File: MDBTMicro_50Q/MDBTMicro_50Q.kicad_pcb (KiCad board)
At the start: 2 copper layers, 33 x 18 mm, 24 parts, among them J1 USB_C_Receptacle_USB2.0, J2 SWD, U1 XC6220B331MR-G, U2 TP4057, U3 MDBT50Q-x1MV2, U4 ProMicro, X1 32.768kHz

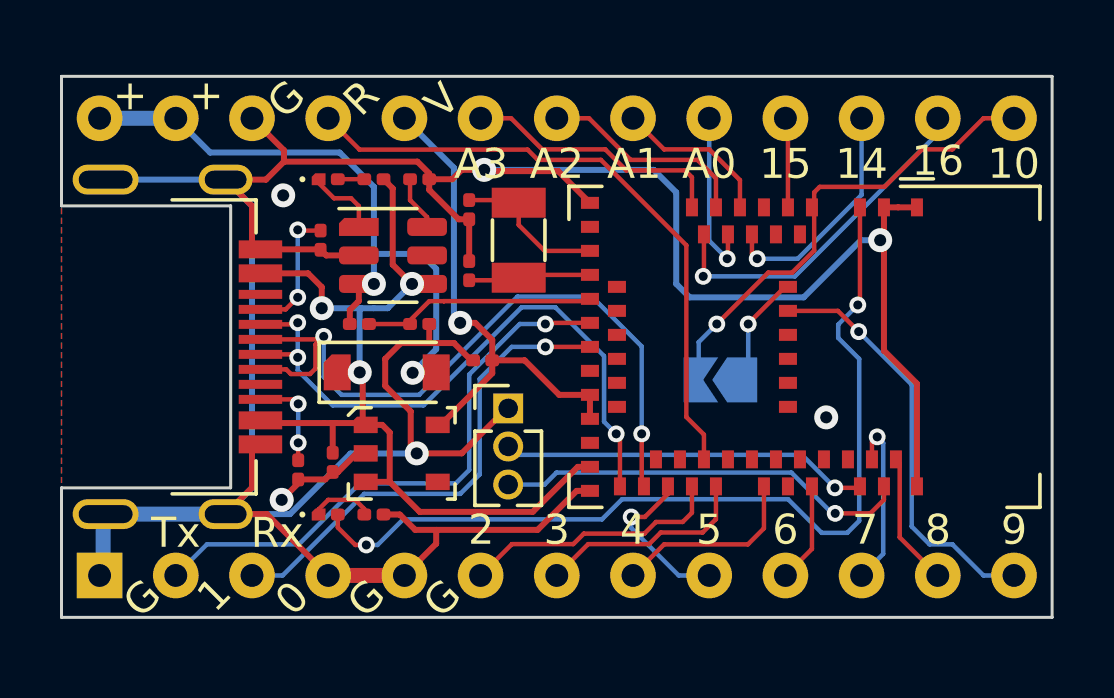
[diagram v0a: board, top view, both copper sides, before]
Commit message: Update footprint
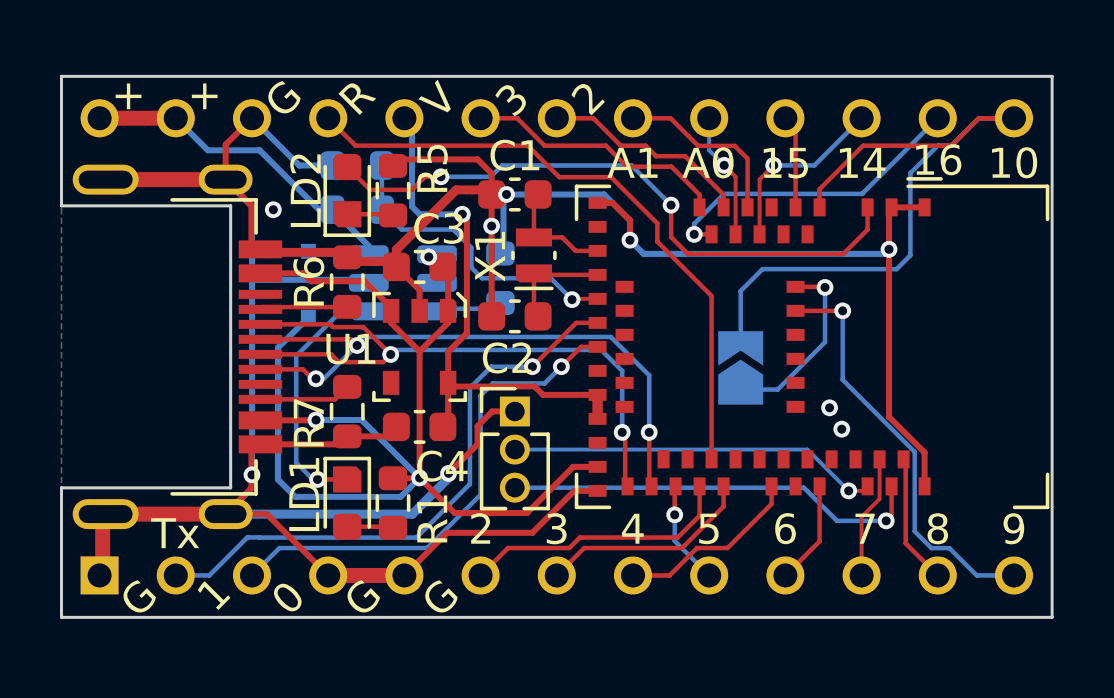
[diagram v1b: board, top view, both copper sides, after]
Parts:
- C1, C2, C3, C4: footprint Capacitor_SMD:C_0201_0603Metric -> Capacitor_SMD:C_0603_1608Metric
- D1: footprint Diode_SMD:D_SOD-123 -> Diode_SMD:D_SOD-323F; moved to B.Cu
- LD1: value RED -> Charging; footprint LED_SMD:LED_0201_0603Metric -> LED_SMD:LED_0603_1608Metric
- LD2: value BLUE -> User; footprint LED_SMD:LED_0201_0603Metric -> LED_SMD:LED_0603_1608Metric
- R1, R5, R6, R7: footprint Resistor_SMD:R_0201_0603Metric -> Resistor_SMD:R_0603_1608Metric
- R2, R3, R4: footprint Resistor_SMD:R_0201_0603Metric -> Resistor_SMD:R_0603_1608Metric; moved to B.Cu
- U2: moved to B.Cu
- X1: footprint Crystal:Crystal_SMD_3215-2Pin_3.2x1.5mm -> Crystal:Crystal_SMD_MicroCrystal_CM9V-T1A-2Pin_1.6x1.0mm
- moved LD1 10.8 mm to (140.3, 106.8), turned to -90 degrees
- moved LD2 10.8 mm to (140.3, 96.4), turned to 90 degrees
- moved R1 10.8 mm to (141.9, 106.8), turned to 90 degrees
- moved R5 10.8 mm to (141.9, 96.4), turned to -90 degrees
- moved C3 7.13 mm to (142.7, 98.9), turned to 0 degrees
- moved R4 5.68 mm to (140.7, 95.6), turned to 0 degrees
- moved R2 4.26 mm to (145.4, 99.3), turned to -90 degrees
- moved D1 3.93 mm to (139.0, 99.5), turned to 90 degrees
- moved R3 3.81 mm to (140.7, 97.0)
- moved U1 3.60 mm to (142.7, 101.6), turned to 180 degrees
- moved C4 3.06 mm to (142.7, 104.3)
- moved R7 2.54 mm to (140.3, 103.8)
- moved C2 2.16 mm to (145.9, 100.6), turned to 0 degrees
- moved R6 1.66 mm to (140.3, 99.4), turned to 90 degrees
- moved C1 1.61 mm to (145.9, 96.5), turned to 0 degrees
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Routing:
- net LED_PIN: track 30.4 -> 20.9 mm
- net VBUS: track 31.6 -> 40.9 mm
- net VBAT: track 22.2 -> 13.1 mm, vias 2 -> 0
- net /P1.11: track 16.1 -> 23.0 mm, vias 1 -> 0
- net Net-(LD1-Pad1): track 2.48 -> 8.57 mm, vias 0 -> 1
- net USB_D+: track 24.9 -> 21.8 mm, vias 2 -> 3
- net BATTERY_PIN: track 7.78 -> 10.4 mm, vias 0 -> 1
- net /P1.04: track 3.79 -> 6.28 mm
- net /P0.13: track 5.42 -> 3.46 mm
- net Net-(J1-PadA5): track 4.73 -> 2.84 mm, vias 2 -> 0
- net /P0.03: track 7.80 -> 6.08 mm
- net /P0.09: track 5.82 -> 4.12 mm, vias 1 -> 0
- net /P0.02: track 5.75 -> 4.23 mm
- net Net-(C1-Pad2): track 5.16 -> 3.80 mm
- net /P0.28: track 11.7 -> 10.5 mm
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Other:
- board text added: "GND SWDIO SWCLK"
- board text removed: "A2"
- board text removed: "A3"
- board text removed: "RST"
- board text removed: "Rx"
- board text removed: "SWCLK"
- board text removed: "SWDIO"
- board text removed: "VDD"
